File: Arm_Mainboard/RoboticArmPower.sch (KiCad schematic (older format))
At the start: 29 parts

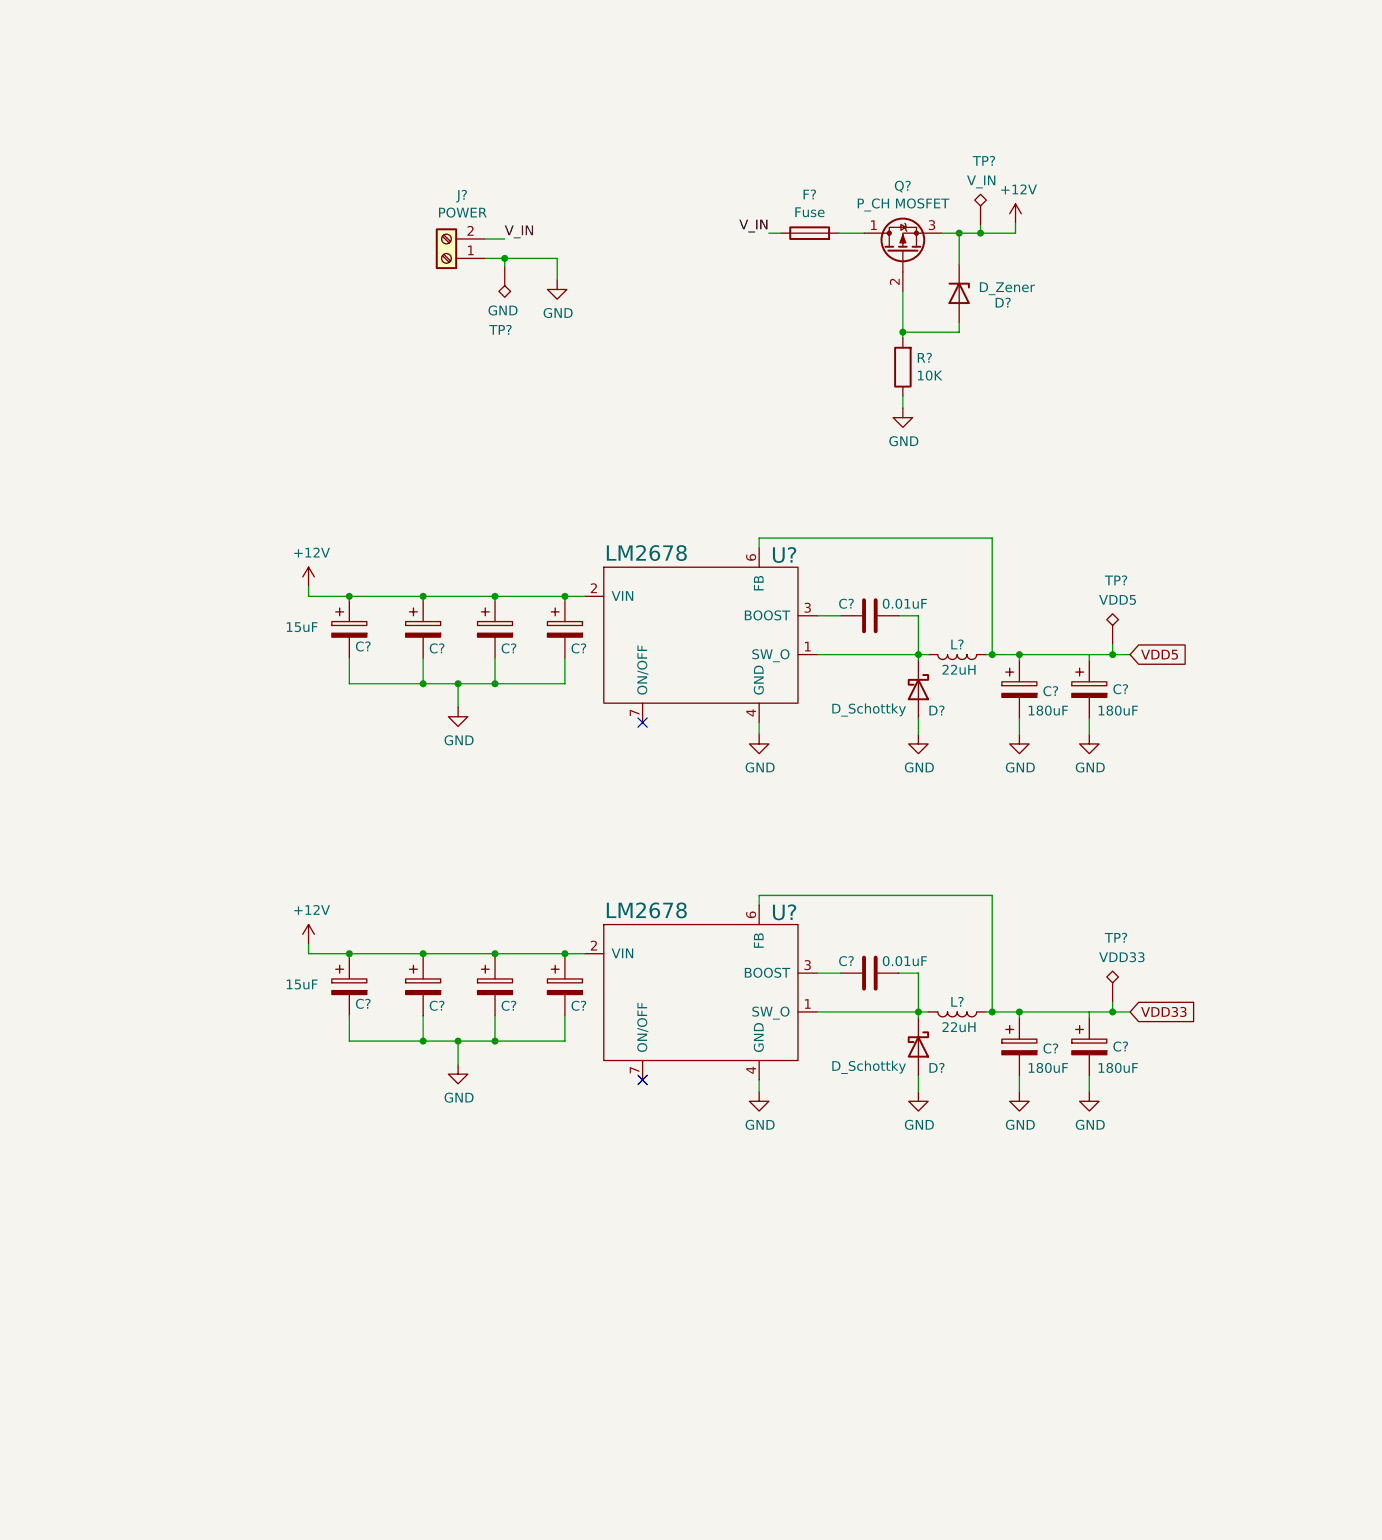
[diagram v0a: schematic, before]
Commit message: PCB
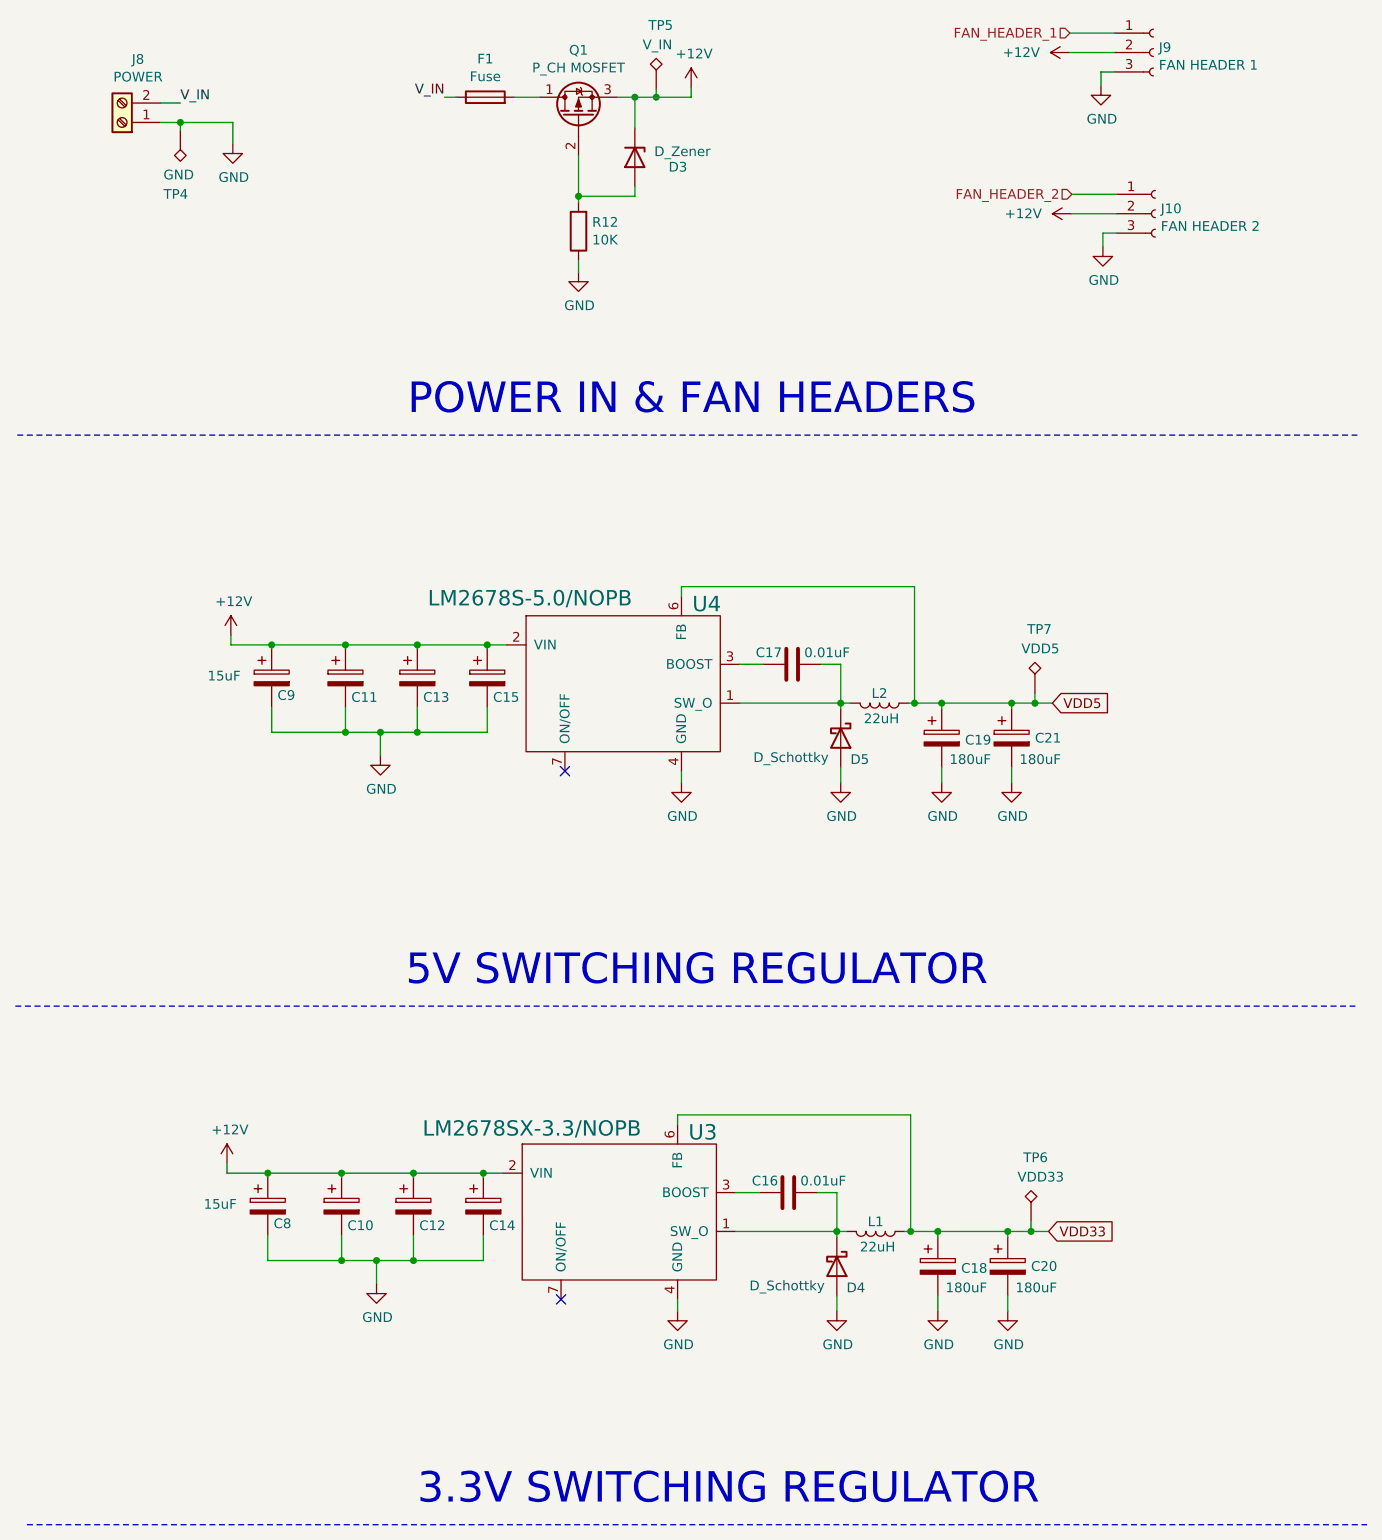
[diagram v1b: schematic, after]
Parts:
- added J10: FAN HEADER 2, Connector_PinHeader_2.54mm:PinHeader_1x03_P2.54mm_Vertical, symbol Connector:Conn_01x03_Female
- added J9: FAN HEADER 1, Connector_PinHeader_2.54mm:PinHeader_1x03_P2.54mm_Vertical, symbol Connector:Conn_01x03_Female
- C10, C11, C12, C13, C14, C15, C8, C9: renamed from C?; footprint (none) -> Capacitor_SMD:CP_Elec_5x5.3
- C16, C17: renamed from C?; footprint (none) -> Capacitor_SMD:C_0805_2012Metric_Pad1.18x1.45mm_HandSolder
- C18, C19, C20, C21: renamed from C?; footprint (none) -> Capacitor_SMD:CP_Elec_6.3x5.9
- J8: renamed from J?; footprint (none) -> ArmFootprints:TerminalBlock_bornier-2_P5.08mmCOPY
- R12: renamed from R?; footprint (none) -> Resistor_SMD:R_0805_2012Metric_Pad1.20x1.40mm_HandSolder
- TP4, TP5, TP6, TP7: renamed from TP?; footprint (none) -> TestPoint:TestPoint_THTPad_3.0x3.0mm_Drill1.5mm
- U3: renamed from U?; value LM2678 -> LM2678SX-3.3/NOPB; footprint (none) -> Package_TO_SOT_SMD:TO-263-7_TabPin4
- U4: renamed from U?; value LM2678 -> LM2678S-5.0/NOPB; footprint (none) -> Package_TO_SOT_SMD:TO-263-7_TabPin4
- gave numbers to parts that had none: 7
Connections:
- net +12V: now also J10.2 (Pin_2), J9.2 (Pin_2)
- net GND: now also J10.3 (Pin_3), J9.3 (Pin_3)
- new net FAN_HEADER_1: J9.1 (Pin_1)
- new net FAN_HEADER_2: J10.1 (Pin_1)
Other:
- note added: "3.3V SWITCHING REGULATOR"
- note added: "5V SWITCHING REGULATOR"
- note added: "POWER IN & FAN HEADERS"
- moved on the sheet: C10, C11, C12, C13, C14, C15, C16, C17, C18, C19, C20, C21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
